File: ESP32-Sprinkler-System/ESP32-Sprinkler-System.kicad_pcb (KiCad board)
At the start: 4 copper layers, 58 parts, among them J101 12V, J102 DHT, J103 NEOPIXEL, J104 LCD, J105 BME280, J201 TBL004-508-02BE-2GY, J202 TBL004-508-02BE-2GY, J203 TBL004-508-02BE-2GY, J204 TBL004-508-02BE-2GY, Q201 IRFZ24NPBF, Q202 IRFZ24NPBF, Q203 IRFZ24NPBF, Q204 IRFZ24NPBF, U101 V7805-500, U102 ESP32-DEVKITC-32D, U201 MC33152PG, U202 MC33152PG

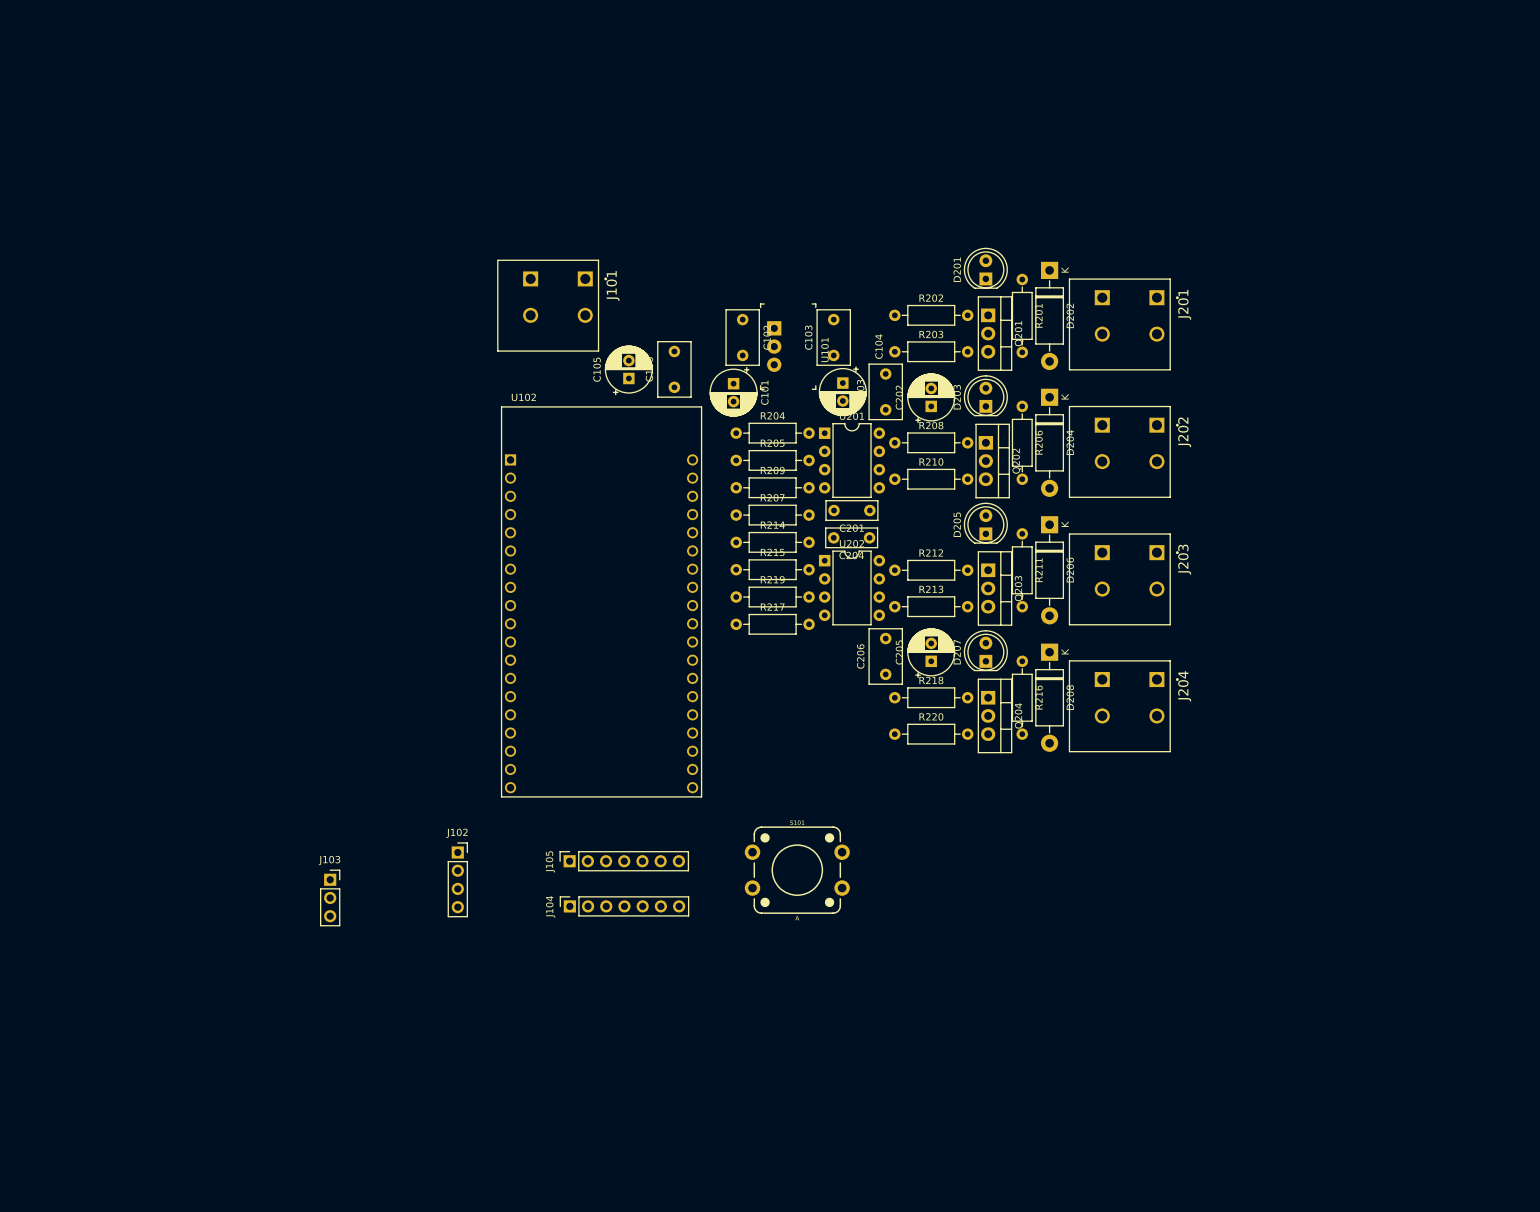
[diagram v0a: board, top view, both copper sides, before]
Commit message: good layout.
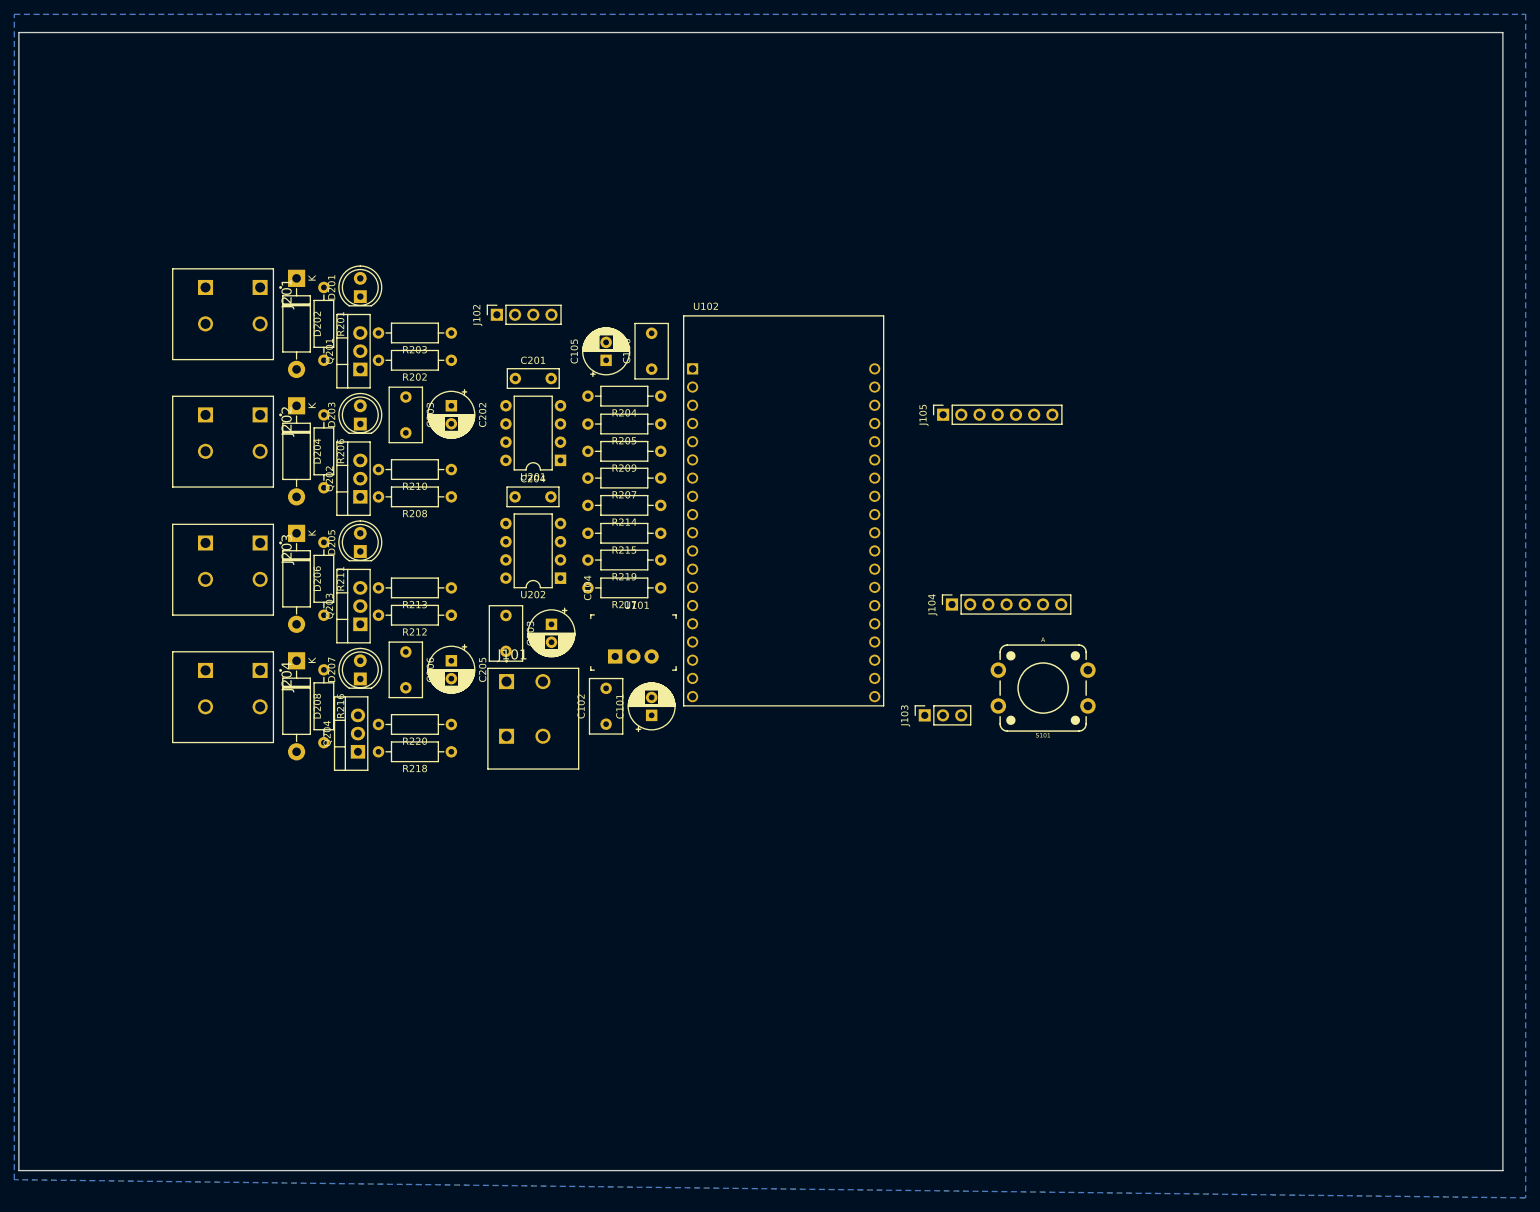
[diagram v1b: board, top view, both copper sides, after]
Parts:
- moved J201 125.1 mm to (70.7, 66.1)
- moved J202 125.1 mm to (70.7, 83.9)
- moved J203 125.1 mm to (70.7, 101.8)
- moved J204 125.1 mm to (70.7, 119.5)
- moved D204 105.0 mm to (75.8, 82.6)
- moved D206 105.0 mm to (75.8, 100.4)
- moved D208 105.0 mm to (75.8, 118.2)
- moved D202 105.0 mm to (75.8, 64.9)
- moved R206 97.4 mm to (79.6, 83.9)
- moved R211 97.4 mm to (79.6, 101.7)
- moved R216 97.4 mm to (79.6, 119.5)
- moved R201 97.4 mm to (79.6, 66.1)
- moved Q204 88.2 mm to (84.4, 130.9), turned to 90 degrees
- moved Q201 87.9 mm to (84.7, 77.6), turned to 90 degrees
- moved Q203 87.9 mm to (84.7, 113.1), turned to 90 degrees
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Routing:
- added copper zone on B.Cu, net GND
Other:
- board outline added: 207 x 158.8 mm
- copper layers 4 -> 2
